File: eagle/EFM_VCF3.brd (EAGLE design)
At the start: 100 x 80 mm, 44 parts, among them IC1 LM13700N, IC2 TL084P, Q3 2N3906, Q4 2N3906, U1 POWER

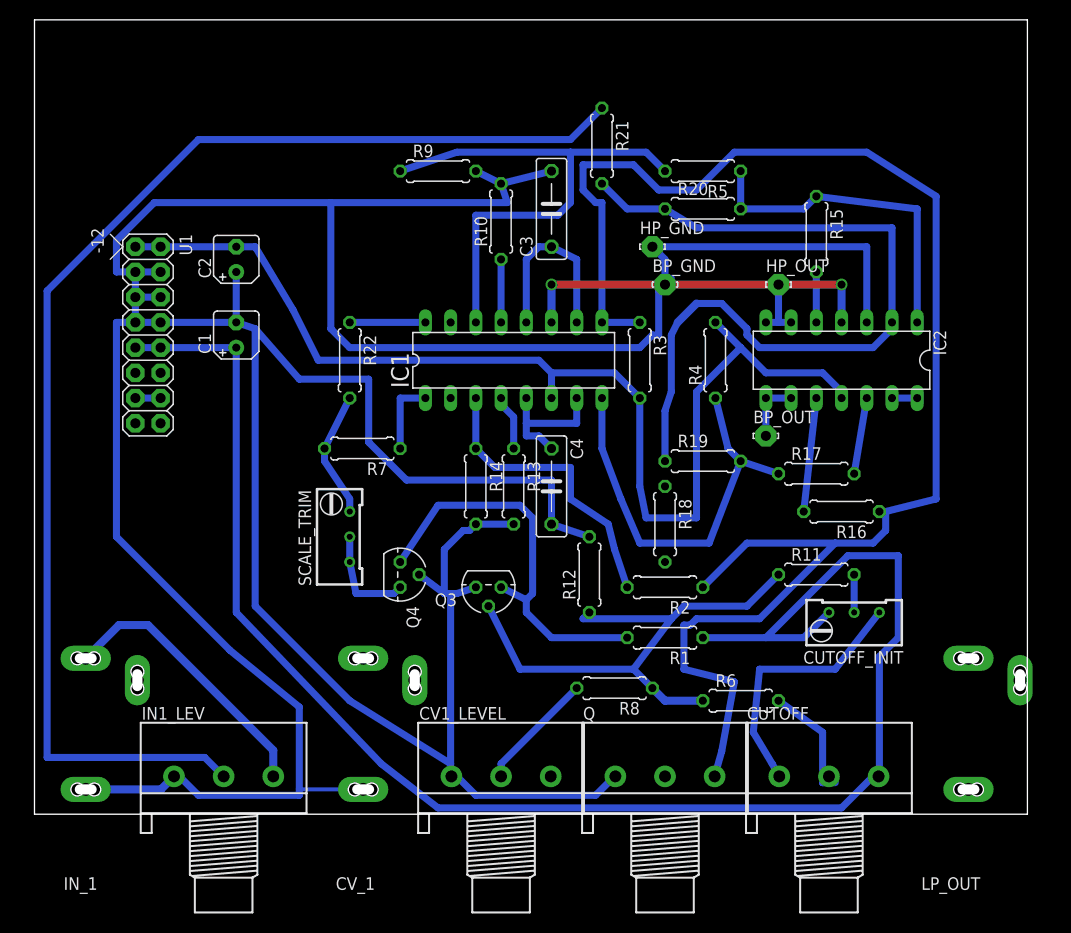
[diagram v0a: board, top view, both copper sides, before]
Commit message: gcode
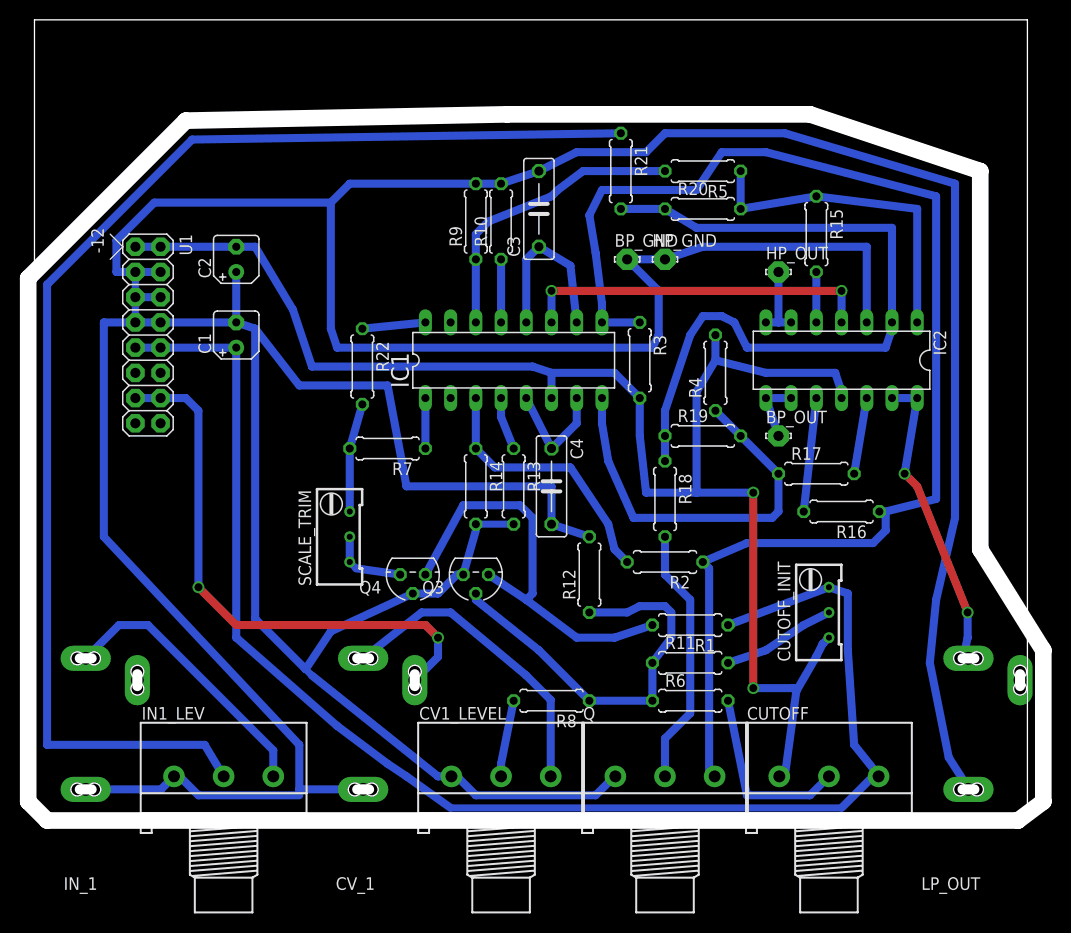
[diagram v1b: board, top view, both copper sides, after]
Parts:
- moved R11 15.5 mm to (66.0, 15.2)
- moved R8 6.48 mm to (52.1, 11.4)
- moved R9 6.35 mm to (44.5, 59.7), turned to 90 degrees
- moved R6 5.08 mm to (66.0, 11.4)
- moved BP_GND 4.58 mm to (59.7, 55.9)
- moved CUTOFF_INIT 4.02 mm to (78.7, 20.3), turned to 0 degrees
- moved R21 3.18 mm to (59.1, 64.8)
- moved R1 2.84 mm to (66.0, 19.1)
- moved R18 2.54 mm to (63.5, 31.8)
- moved R19 2.54 mm to (67.3, 38.1)
- moved R2 2.54 mm to (63.5, 25.4)
- moved R7 2.54 mm to (35.6, 36.8)
- moved HP_GND 1.80 mm to (63.5, 55.9)
- moved Q3 1.80 mm to (44.5, 24.1)
- moved R22 1.42 mm to (33.0, 45.1)
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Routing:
- net GND: track 414.7 -> 511.2 mm
- net N$55: track 2.54 -> 56.1 mm, vias 0 -> 2
- net N$54: track 0.00 -> 31.5 mm
- net N$14: track 2.54 -> 30.9 mm, vias 0 -> 2
- net N$19: track 0.00 -> 26.2 mm
- net N$4: track 53.7 -> 29.9 mm
- net N$5: track 157.4 -> 133.8 mm
- net N$38: track 164.5 -> 143.7 mm
- net N$18: track 55.6 -> 40.5 mm
- net -12V: track 140.5 -> 153.5 mm, vias 0 -> 2
- net N$27: track 3.81 -> 11.4 mm
- net N$56: track 12.7 -> 18.8 mm
- net N$26: track 80.6 -> 75.5 mm
- net N$10: track 12.0 -> 7.75 mm
- net N$6: track 29.8 -> 26.7 mm
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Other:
- board size 100 x 80 mm -> 102.2 x 80.6 mm
